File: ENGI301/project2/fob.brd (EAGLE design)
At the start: 101.6 x 100 mm, 21 parts, among them SW1 PUSH_BUTTON, SW2 PUSH_BUTTON, SW3 PUSH_BUTTON, SW4 PUSH_BUTTON

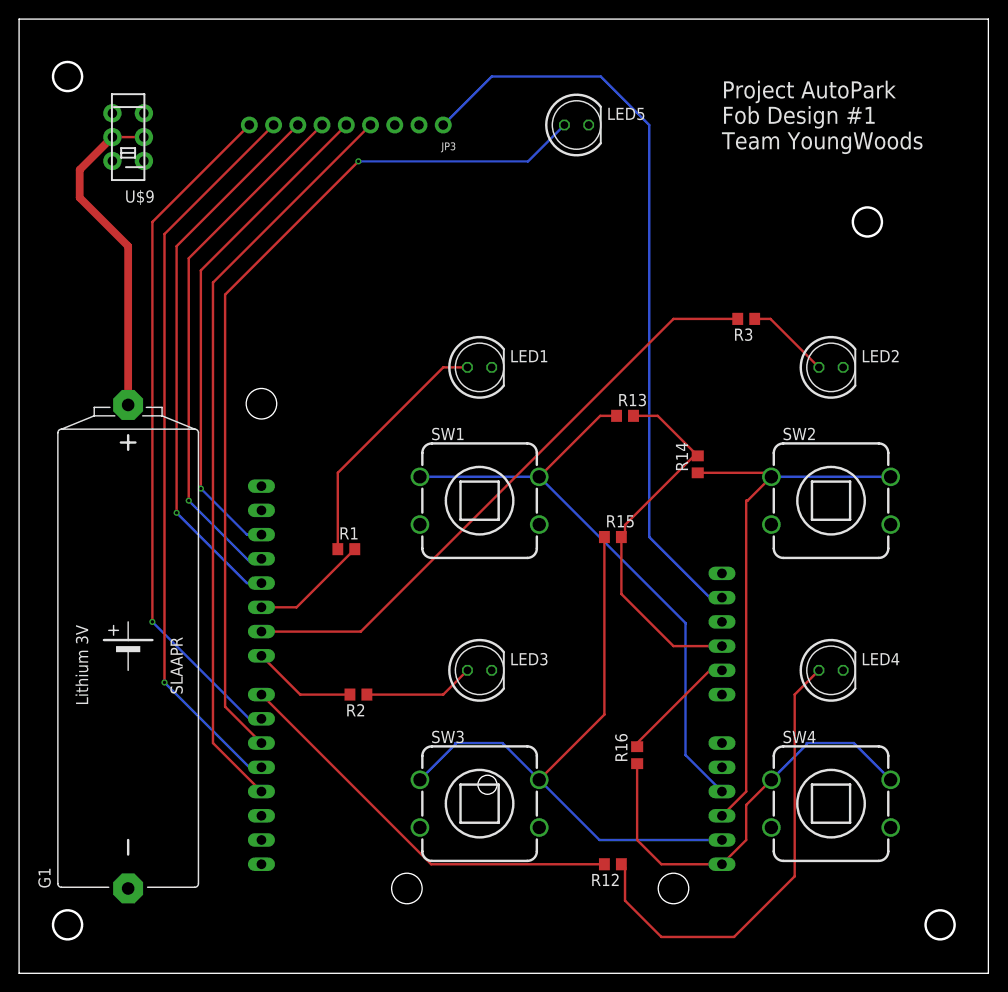
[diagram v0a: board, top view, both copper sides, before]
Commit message: Added gbr files
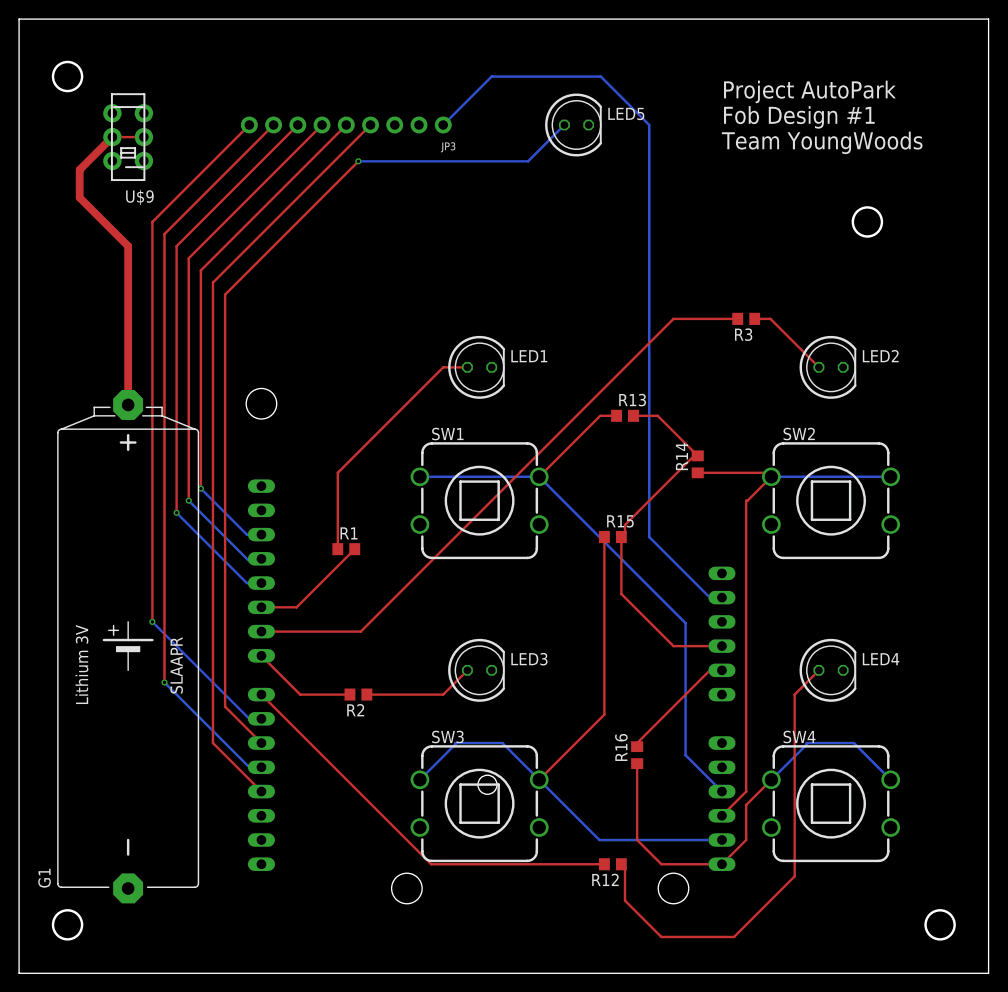
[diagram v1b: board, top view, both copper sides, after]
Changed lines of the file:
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@@
 <board>
 <plain>
-<wire x1="0" y1="0" x2="101.58" y2="0" width="0" layer="20"/>
-<wire x1="101.58" y1="0" x2="101.58" y2="100" width="0" layer="20"/>
-<wire x1="101.58" y1="100" x2="0" y2="100" width="0" layer="20"/>
+<wire x1="0" y1="0" x2="101.6" y2="0" width="0" layer="20"/>
+<wire x1="101.6" y1="0" x2="101.6" y2="100" width="0" layer="20"/>
+<wire x1="101.6" y1="100" x2="0" y2="100" width="0" layer="20"/>
 <wire x1="0" y1="100" x2="0" y2="0" width="0" layer="20"/>
 <text x="73.66" y="86.36" size="1.778" layer="21">Project AutoPark
@@
 <dimension x1="6.604" y1="5.08" x2="3.556" y2="5.08" x3="5.08" y3="2.54" textsize="1.778" layer="1" dtype="diameter"/>
 <dimension x1="94.996" y1="5.08" x2="98.044" y2="5.08" x3="96.52" y3="7.62" textsize="1.778" layer="1" dtype="diameter"/>
-<dimension x1="39.37" y1="6.35" x2="39.37" y2="74.93" x3="-5.08" y3="40.64" textsize="1.778" layer="20"/>
-<dimension x1="11.43" y1="59.563" x2="11.43" y2="8.89" x3="0" y3="34.2265" textsize="1.778" layer="20"/>
 </plain>
 <attributes>
